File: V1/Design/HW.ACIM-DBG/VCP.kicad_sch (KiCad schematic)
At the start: 49 parts, among them Q1 MFET N, U10 12MHz, U3 SPI EEPROM, U8 FT4232H, U9 SHIFT REG 8BIT

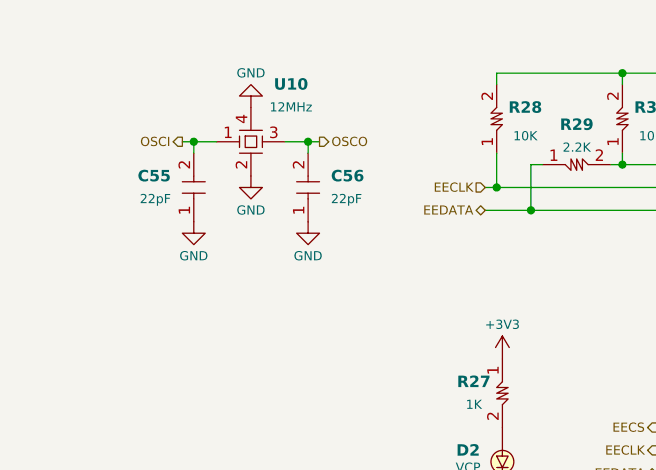
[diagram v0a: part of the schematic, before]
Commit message: Production HW.ACIM-DBG_V1.0 update BoM
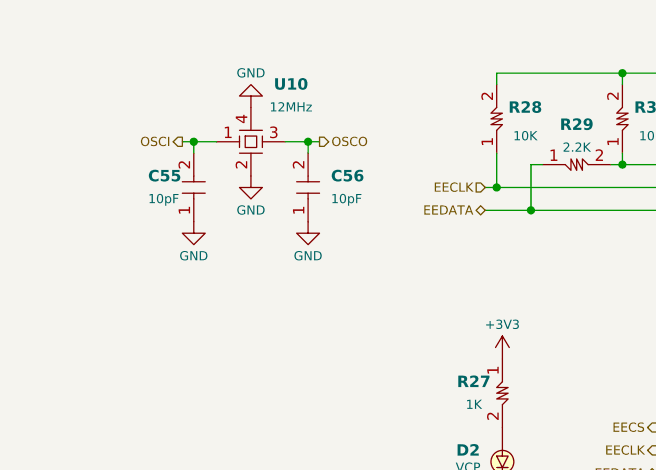
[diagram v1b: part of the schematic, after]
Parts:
- C55, C56: value 22pF -> 10pF; MNP CC0603JRNPO9BN220 -> CC0603JRNPO9BN100
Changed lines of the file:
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@@
 (kicad_sch
-	(version 20231120)
+	(version 20250114)
 	(generator "eeschema")
-	(generator_version "8.0")
+	(generator_version "9.0")
 	(paper "A4")
 	(title_block
@@
 		(on_board yes)
 		(dnp no)
-		(fields_autoplaced yes)
 		(property "Reference" "C55"
-			(at 41.91 44.4499 90)
+			(at 39.37 44.45 90)
 			(effects
 				(font
@@
 					(bold yes)
 				)
-				(justify right)
+				(justify left)
 			)
 		)
-		(property "Value" "22pF"
-			(at 41.91 46.9899 90)
+		(property "Value" "10pF"
+			(at 39.37 46.9899 90)
 			(effects
 				(font
@@
 					(thickness 0.254)
 				)
-				(justify right)
+				(justify left)
 			)
 		)
@@
 			)
 		)
-		(property "Description" "CAP CER SMD 0603 22pF 50V 5% NP0 WxLxH(0x1.6x0.9)"
+		(property "Description" "CAP CER SMD 0603 10pF 50V 5% NP0 WxLxH(0x1.6x0.9)"
 			(at 46.99 46.99 0)
 			(effects
@@
 			)
 		)
-		(property "MNP" "CC0603JRNPO9BN220"
+		(property "MNP" "CC0603JRNPO9BN100"
 			(at 46.99 46.99 0)
 			(effects
@@
 		(fields_autoplaced yes)
 		(property "Reference" "C56"
-			(at 59.69 44.4499 90)
+			(at 59.69 44.45 90)
 			(effects
 				(font
@@
 			)
 		)
-		(property "Value" "22pF"
+		(property "Value" "10pF"
 			(at 59.69 46.9899 90)
 			(effects
@@
 			)
 		)
-		(property "Description" "CAP CER SMD 0603 22pF 50V 5% NP0 WxLxH(0x1.6x0.9)"
+		(property "Description" "CAP CER SMD 0603 10pF 50V 5% NP0 WxLxH(0x1.6x0.9)"
 			(at 54.61 46.99 0)
 			(effects
@@
 			)
 		)
-		(property "MNP" "CC0603JRNPO9BN220"
+		(property "MNP" "CC0603JRNPO9BN100"
 			(at 54.61 46.99 0)
 			(effects
